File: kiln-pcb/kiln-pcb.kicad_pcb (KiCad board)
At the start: 2 copper layers, 91.4 x 55.9 mm, 12 parts, among them J1 TFT, J2 TEMP, J3 ROTARY, J4 Relay, U1 WeMos_D1_mini

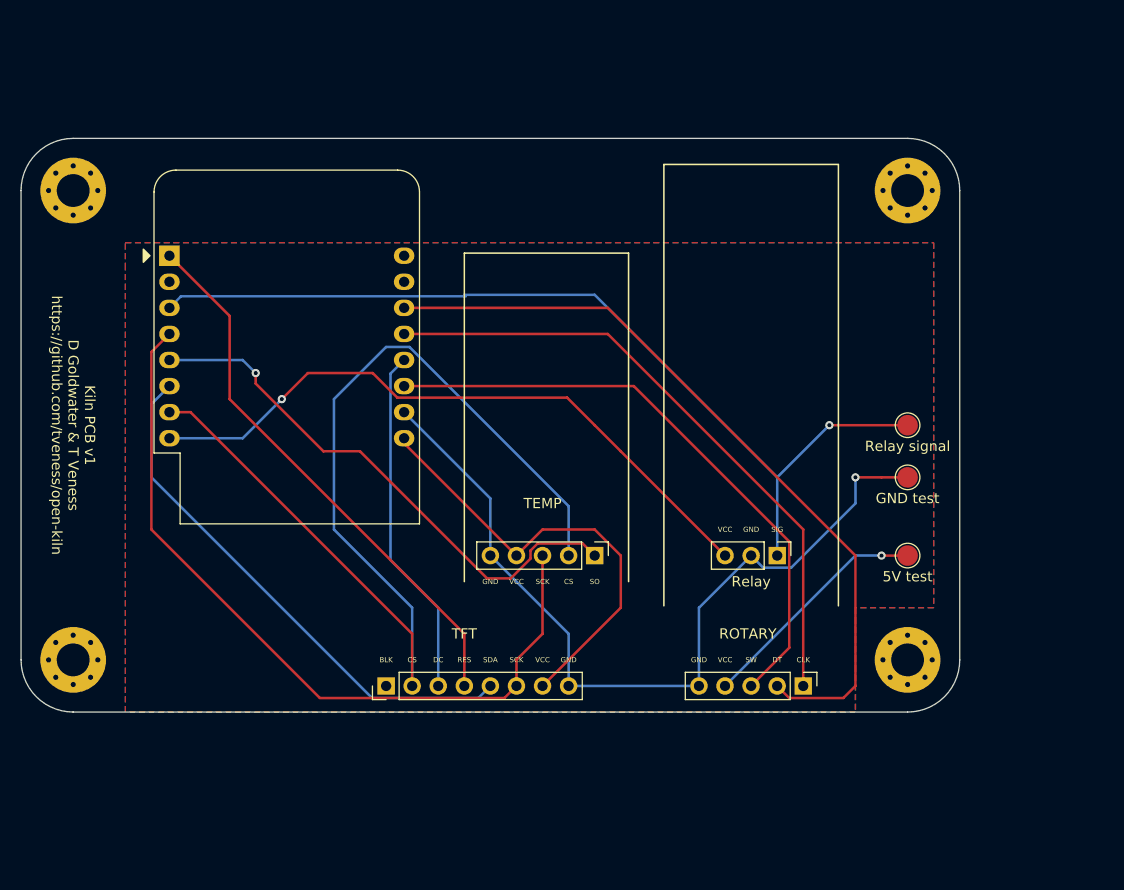
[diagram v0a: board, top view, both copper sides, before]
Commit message: PCB v1.1
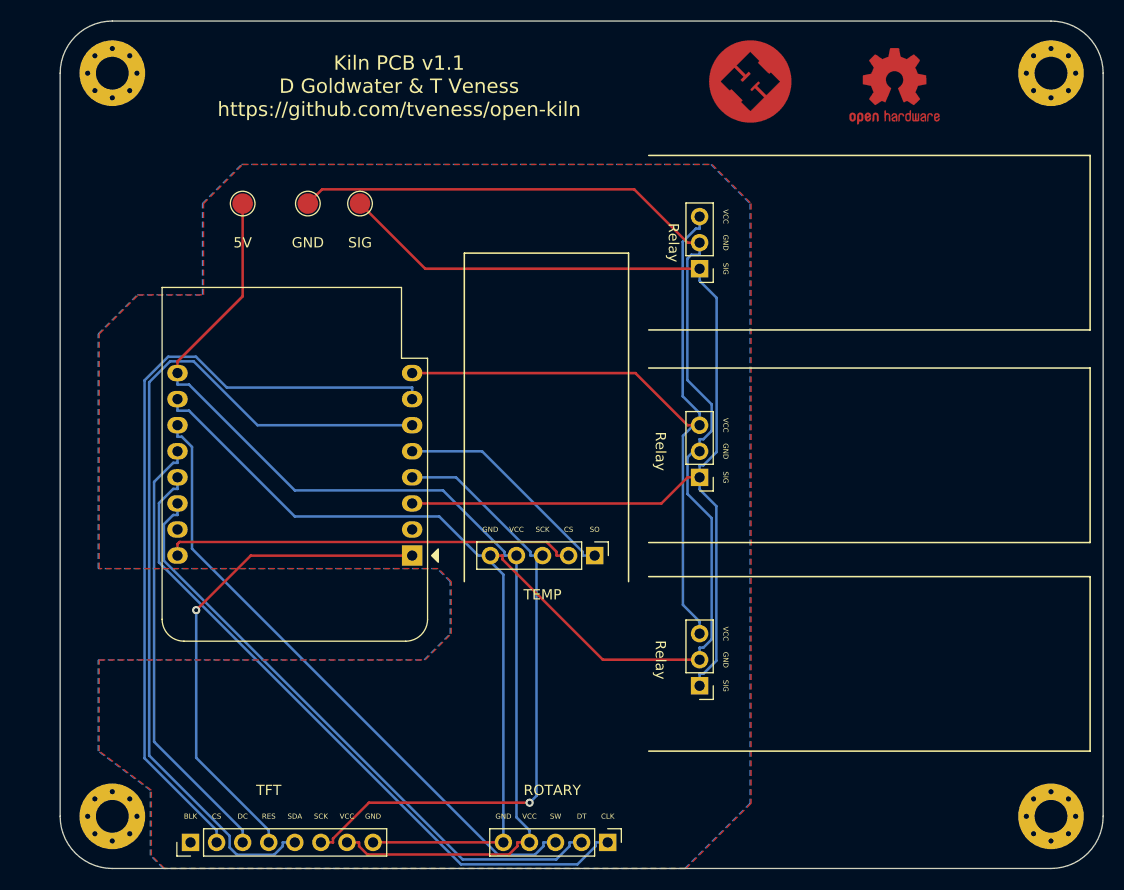
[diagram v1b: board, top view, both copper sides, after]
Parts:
- added J5: Relay, Connector_PinHeader_2.54mm:PinHeader_1x03_P2.54mm_Vertical, F.Cu at (137.2, 83.8)
- added J6: Relay, Connector_PinHeader_2.54mm:PinHeader_1x03_P2.54mm_Vertical, F.Cu at (137.2, 104.1)
- added REF**: OSHW-Logo2_9.8x8mm_Copper, Symbol:OSHW-Logo2_9.8x8mm_Copper, F.Cu at (156.2, 45.7)
- added Ref**: Val**, wemos_d1_mini:hackspace_small, F.Cu at (141.0, 44.5)
- TP1: value 5V test -> 5V
- TP2: value GND test -> GND
- TP3: value Relay signal -> SIG
- moved TP1 73.3 mm to (92.7, 57.1)
- moved TP2 64.2 mm to (99.1, 57.1)
- moved TP3 57.5 mm to (104.1, 57.1)
- moved U1 37.6 mm to (109.2, 91.4), turned to 180 degrees
- moved J4 28.9 mm to (137.2, 63.5), turned to 180 degrees
- moved J1 24.4 mm to (87.6, 119.4)
- moved J3 24.4 mm to (128.3, 119.4)
- moved H1 20.7 mm to (171.4, 116.8)
- moved H2 18.1 mm to (171.4, 44.5)
- moved H3 15.7 mm to (80.0, 116.8)
- moved H4 12.0 mm to (80.0, 44.5)
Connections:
- J1 pad 2: CS_T -> CS_TFT
- U1 pad 16: unconnected-(U1-Pad16) -> CS_T
- U1 pad 7: CS_T -> CS_TFT
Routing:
- net GND_ROTARY: track 81.7 -> 190.6 mm, vias 1 -> 0
- net CS_TFT: track 0.00 -> 77.3 mm
- net CS_T: track 105.0 -> 40.1 mm
- net VCC_ROTARY: track 67.1 -> 108.0 mm, vias 1 -> 0
- net SDA_TFT: track 52.0 -> 85.0 mm
- net SO_T: track 53.2 -> 22.2 mm, vias 1 -> 0
- net Sig_relay: track 89.6 -> 108.5 mm, vias 1 -> 0
- net DT_ROTARY: track 75.3 -> 60.0 mm
- net SCK_T: track 76.4 -> 62.6 mm, vias 0 -> 1
- net Vcc_relay: track 64.1 -> 74.2 mm, vias 1 -> 0
- net DC_TFT: track 34.2 -> 42.9 mm
- net RES_TFT: track 53.8 -> 48.8 mm, vias 0 -> 1
- net CLK_ROTARY: track 62.0 -> 66.3 mm
- net SW_ROTARY: track 59.4 -> 61.3 mm
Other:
- board size 91.4 x 55.9 mm -> 101.6 x 82.6 mm
- board text added: "Kiln PCB v1.1 D Goldwater & T Veness https://github.com/tveness/open-kiln"
- board text removed: "Kiln PCB v1 D Goldwater & T Veness https://github.com/tveness/open-kiln"
